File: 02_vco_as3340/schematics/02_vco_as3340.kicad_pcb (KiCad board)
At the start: 2 copper layers, 62.5 x 111.8 mm, 89 parts, among them J1 Header 1, J10 SINE OUT, J2 Header 2, J3 SYNC IN, J4 FM IN, J5 PWM CV IN, J6 1V per O IN, J7 SQUARE OUT, J8 SAW OUT, J9 TRI OUT, Q1 BC547C, Q2 BC547C, U1 TL072, U2 AS3340, U3 TL074

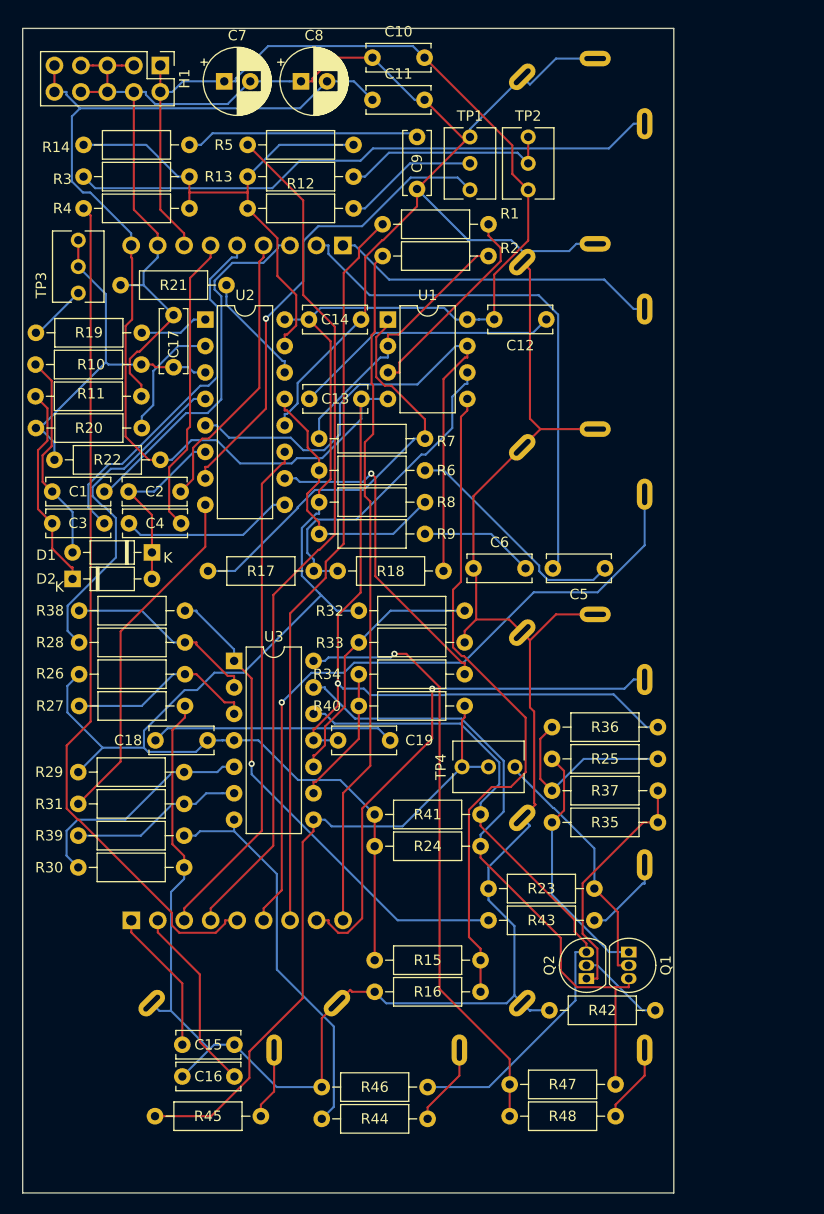
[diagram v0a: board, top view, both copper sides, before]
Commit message: routed everyting
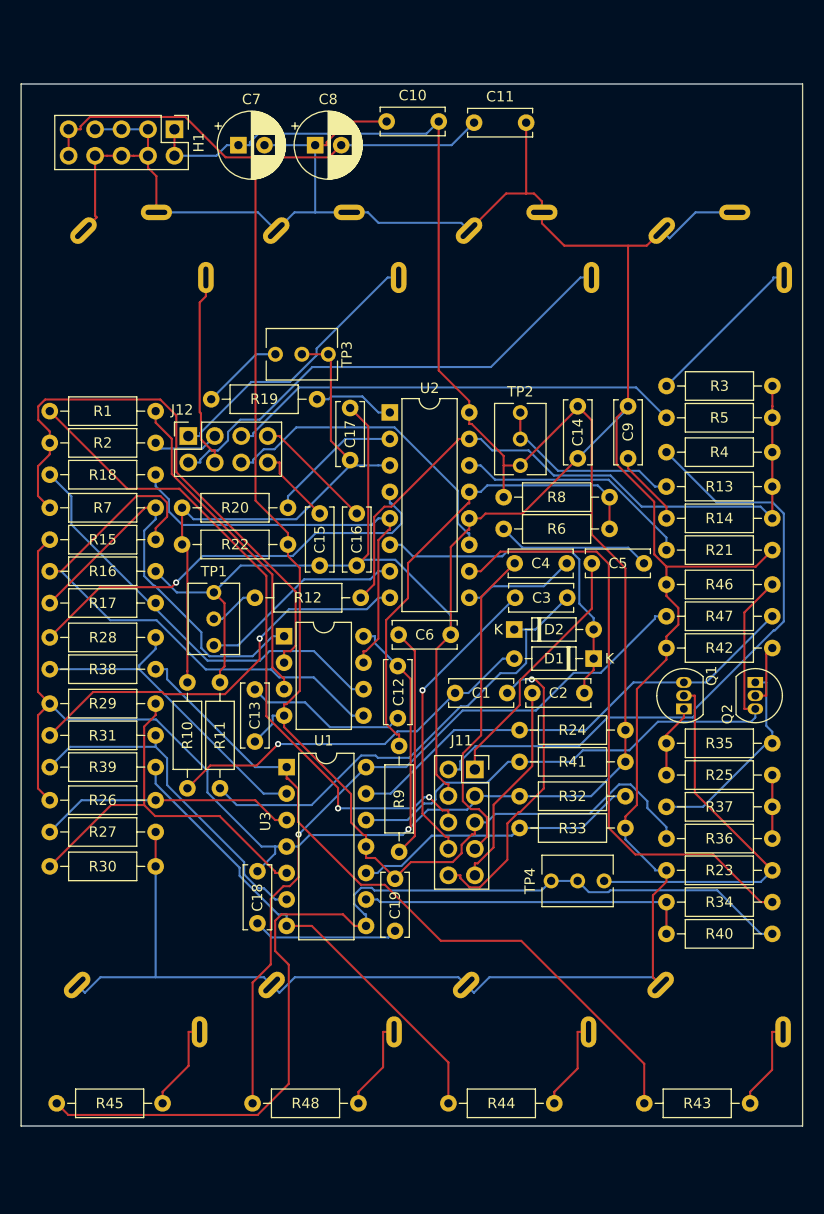
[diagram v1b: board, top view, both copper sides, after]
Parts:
- removed J1: Header 1, Connector_PinHeader_2.54mm:PinHeader_1x09_P2.54mm_Vertical
- removed J2: Header 2, Connector_PinHeader_2.54mm:PinHeader_1x09_P2.54mm_Vertical
- added J11: Header 1, Connector_PinSocket_2.54mm:PinSocket_2x05_P2.54mm_Vertical, F.Cu at (188.3, 109.3)
- added J12: Header 2, Connector_PinSocket_2.54mm:PinSocket_2x04_P2.54mm_Vertical, F.Cu at (160.8, 77.3)
- moved R14 75.2 mm to (216.9, 85.2), turned to 180 degrees
- moved R21 67.5 mm to (216.9, 88.2), turned to 180 degrees
- moved R4 60.6 mm to (206.7, 78.8)
- moved R3 59.4 mm to (206.7, 72.5)
- moved R46 58.5 mm to (216.9, 91.5)
- moved R13 58.5 mm to (216.9, 82.1), turned to 180 degrees
- moved C15 52.7 mm to (173.4, 84.7), turned to -90 degrees
- moved C16 51.8 mm to (177.0, 89.7), turned to 90 degrees
- moved R15 51.0 mm to (147.5, 87.2)
- moved TP1 50.2 mm to (163.3, 92.3)
- moved C3 49.9 mm to (197.2, 92.8), turned to 180 degrees
- moved R5 48.0 mm to (206.7, 75.5)
- moved C2 47.8 mm to (198.8, 101.9), turned to 180 degrees
- moved R47 47.4 mm to (216.9, 94.6)
- moved R16 45.5 mm to (157.7, 90.3), turned to 180 degrees
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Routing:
- net PWM CV Levelled: track 65.9 -> 6.39 mm
- net GND: track 341.6 -> 388.8 mm
- net Net-(J6-T): track 56.9 -> 15.7 mm
- net Sync COM: track 67.6 -> 27.0 mm, vias 1 -> 0
- net Fine Tuning: track 82.9 -> 44.1 mm
- net Net-(R40-Pad2): track 63.3 -> 96.3 mm
- net Net-(U1A--): track 25.9 -> 54.6 mm
- net Net-(U2-VTO): track 31.9 -> 58.6 mm, vias 1 -> 0
- net FM CV Levelled: track 51.0 -> 24.4 mm
- net Net-(U2-VHFT): track 45.8 -> 19.8 mm, vias 1 -> 0
- net Net-(D2-K): track 19.8 -> 45.4 mm
- net Net-(R38-Pad2): track 47.5 -> 69.5 mm, vias 1 -> 0
- net +12V: track 211.2 -> 231.0 mm, vias 0 -> 1
- net Net-(U2-VLFI): track 26.8 -> 45.7 mm
- net Net-(U3C--): track 13.4 -> 32.0 mm
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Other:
- board size 62.5 x 111.8 mm -> 75 x 100 mm
